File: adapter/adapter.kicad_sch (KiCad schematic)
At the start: 11 parts, among them J1 AudioJack4, J2 AudioJack4, J3 Conn_01x02_Female, J4 Conn_01x03_Female, J5 Conn_01x03_Female, J6 Conn_01x02_Female, J7 Conn_01x06_Female, SW1 SW_SPST, SW2 SW_SPST, U1 ProMicro, U2 ProMicro

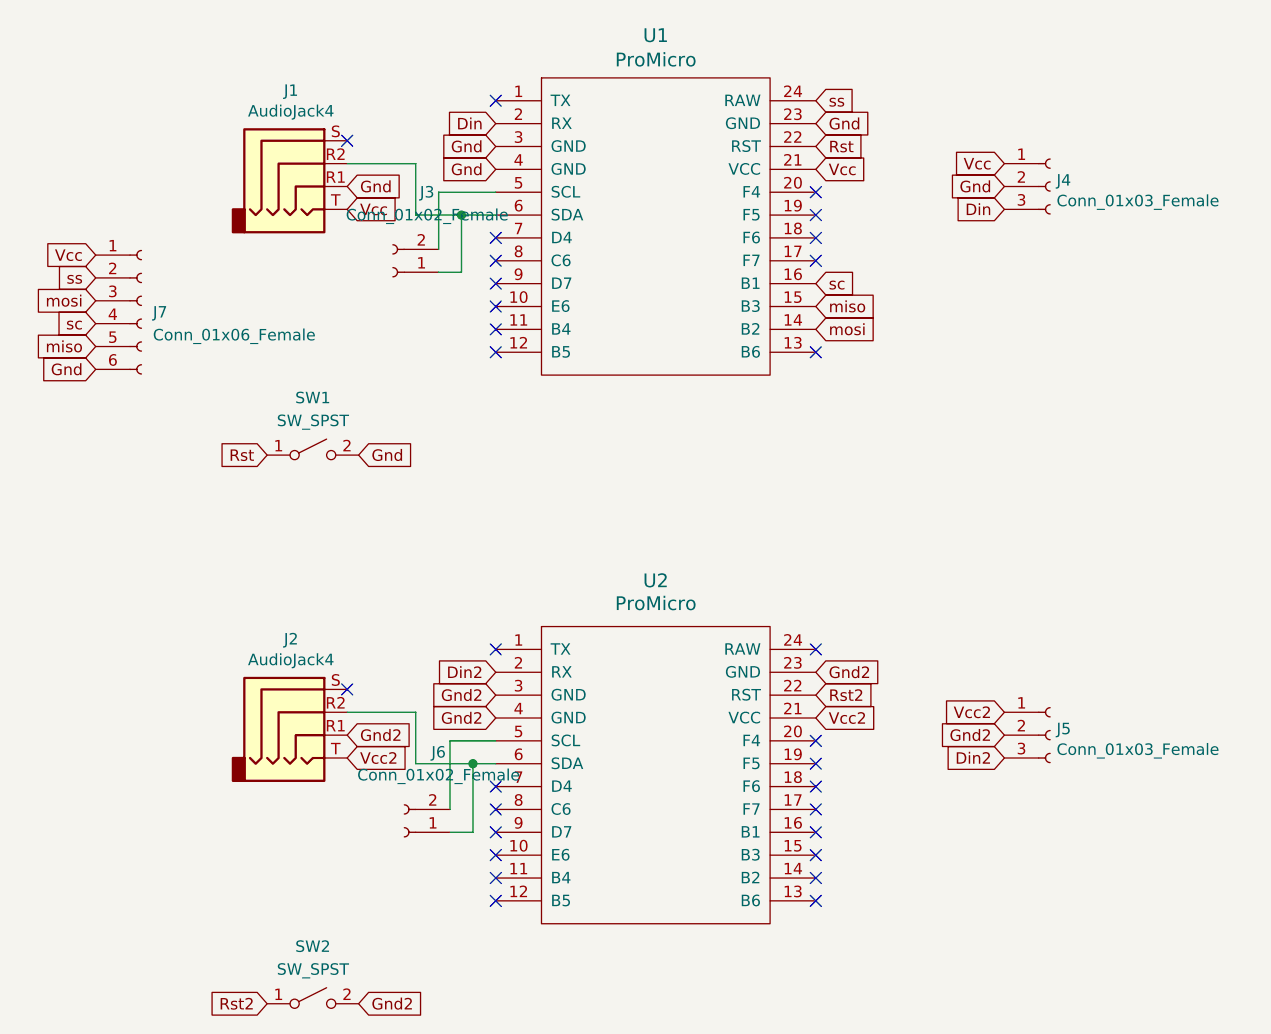
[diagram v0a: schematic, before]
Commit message: left adapter
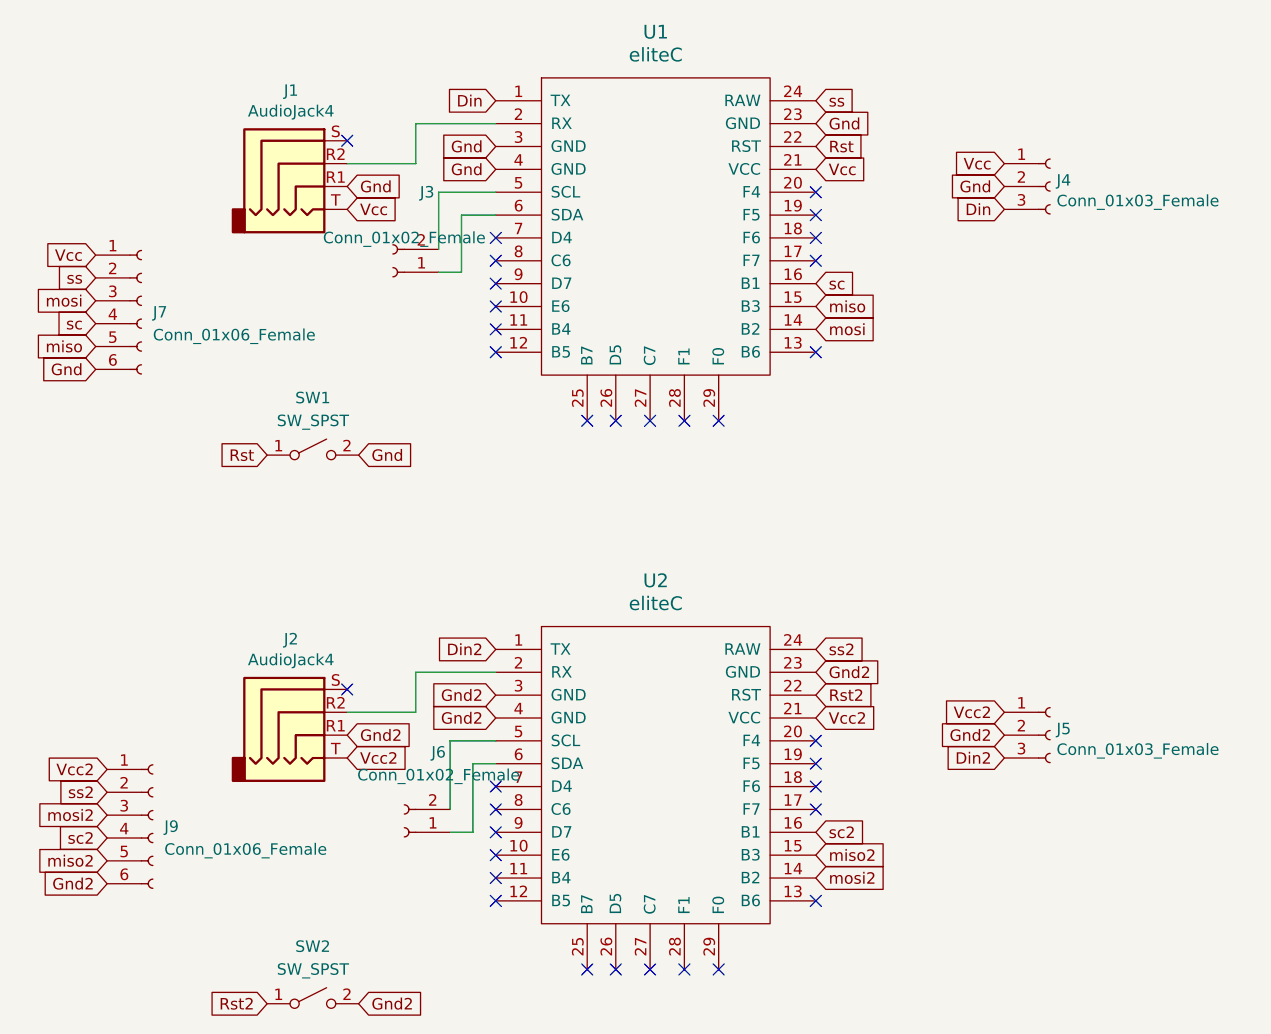
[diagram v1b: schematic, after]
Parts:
- removed U1, U2: ProMicro, Library:Elite-C-castellated-29pin-holes, symbol promicro:ProMicro
- added J9: Conn_01x06_Female, Connector_PinHeader_2.54mm:PinHeader_1x06_P2.54mm_Vertical, symbol Connector:Conn_01x06_Female
- added U1, U2: eliteC, Library:Elite-C-castellated-29pin-holes, symbol elite-C:eliteC
- J7: footprint (none) -> Connector_PinHeader_2.54mm:PinHeader_1x06_P2.54mm_Vertical
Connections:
- net Din: now also U1.1 (TX)
- net Din2: now also U2.1 (TX)
- net Gnd: now also U1.23 (GND), U1.3 (GND), U1.4 (GND)
- net Gnd2: now also J9.6 (Pin_6), U2.23 (GND), U2.3 (GND), U2.4 (GND)
- net Rst: now also U1.22 (RST)
- net Rst2: now also U2.22 (RST)
- net Vcc: now also U1.21 (VCC)
- net Vcc2: now also J9.1 (Pin_1), U2.21 (VCC)
- net miso: now also U1.15 (B3)
- net mosi: now also U1.14 (B2)
- net sc: now also U1.16 (B1)
- net ss: now also U1.24 (RAW)
- net at J6.1 (Pin_1): now also U2.6 (SDA); no longer J2.R2
- net at J6.2 (Pin_2): now also U2.5 (SCL)
- net at J1.R2: now also U1.2 (RX); no longer J3.1 (Pin_1)
- net at J3.2 (Pin_2): now also U1.5 (SCL)
- new net: J3.1 (Pin_1), U1.6 (SDA)
- new net: J2.R2, U2.2 (RX)
- new net miso2: J9.5 (Pin_5), U2.15 (B3)
- new net mosi2: J9.3 (Pin_3), U2.14 (B2)
- new net sc2: J9.4 (Pin_4), U2.16 (B1)
- new net ss2: J9.2 (Pin_2), U2.24 (RAW)
- no-connect marks 30 -> 34
